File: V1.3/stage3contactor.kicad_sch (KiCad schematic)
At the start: 9 parts, among them J10 Screw_Terminal_01x02, J11 Screw_Terminal_01x02, J12 Screw_Terminal_01x02, J14 Screw_Terminal_01x02, J5 Screw_Terminal_01x02, J6 Screw_Terminal_01x02, J7 Screw_Terminal_01x02, J8 Screw_Terminal_01x02, J9 Screw_Terminal_01x02

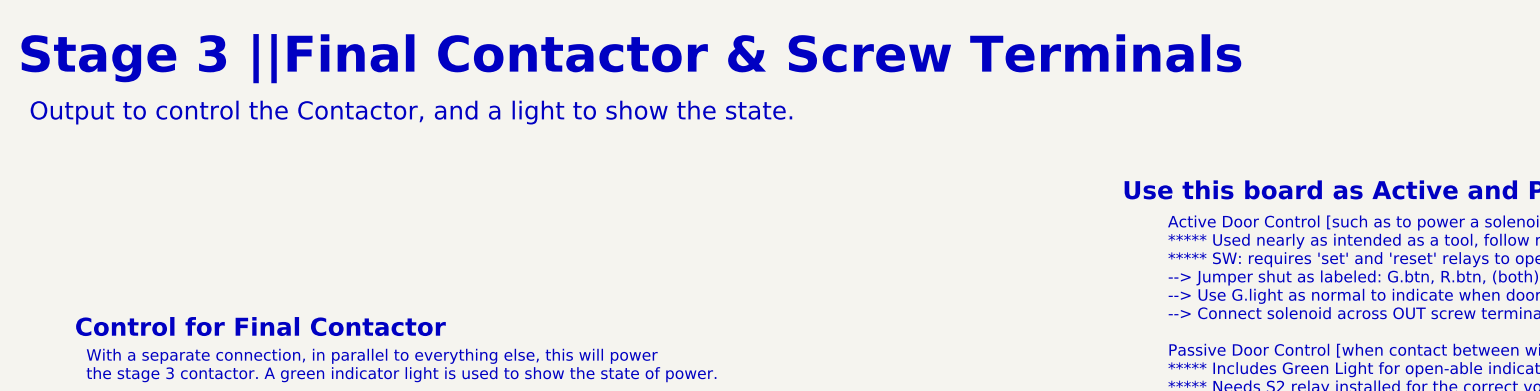
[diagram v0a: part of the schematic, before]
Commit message: update v1.3 schematic documentation
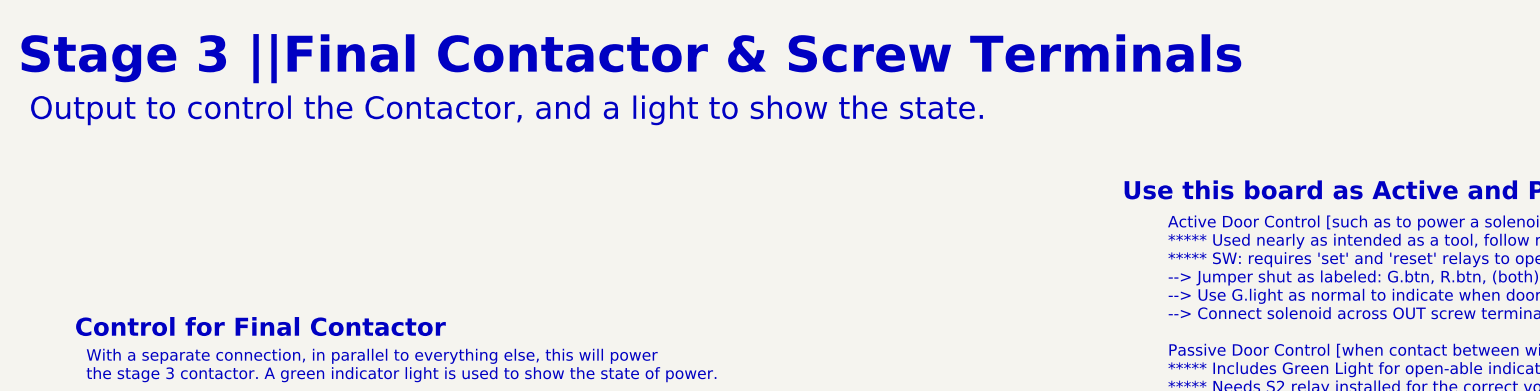
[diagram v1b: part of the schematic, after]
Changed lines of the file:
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@@
   (text "Output to control the Contactor, and a light to show the state."
     (at 36.83 35.56 0)
-    (effects (font (size 2 2)) (justify left bottom))
+    (effects (font (size 2.5 2.5)) (justify left bottom))
   )
   (text "N-ON switch\nneeded for bypass mode" (at 92.71 132.08 0)
